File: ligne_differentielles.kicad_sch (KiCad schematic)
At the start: 2 parts, among them U16 AM26LS32ACDR

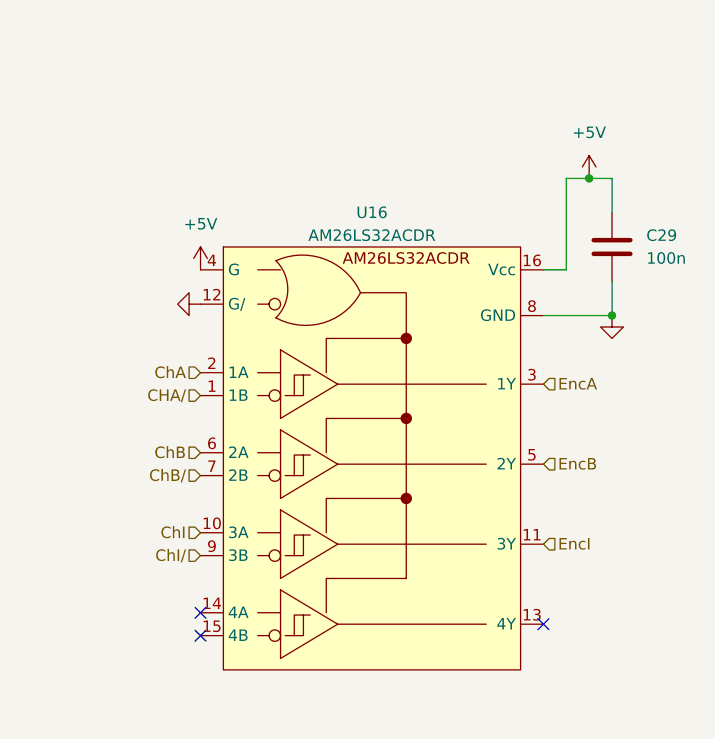
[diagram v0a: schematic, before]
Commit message: finalisation PCB
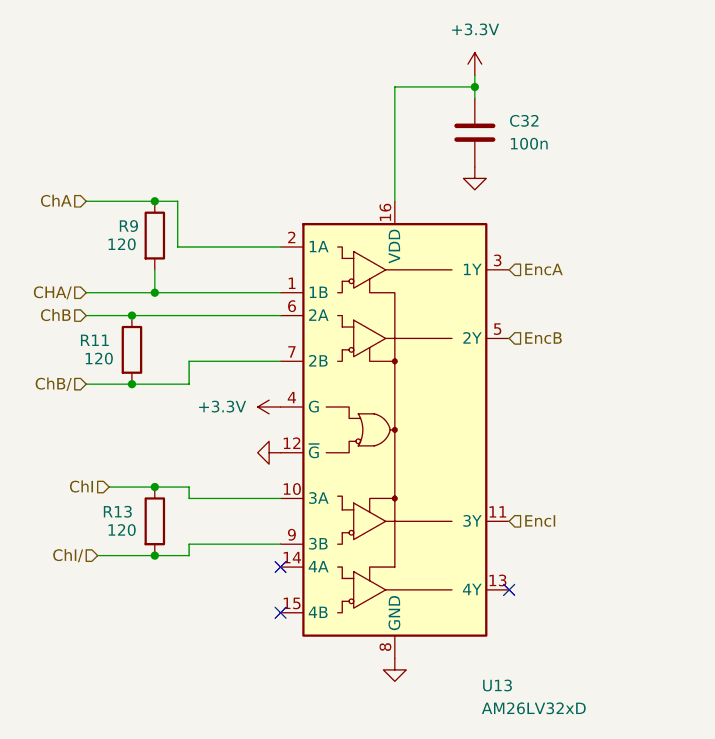
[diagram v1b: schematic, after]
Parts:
- removed C29: 100n, Capacitor_SMD:C_0402_1005Metric, symbol Device:C
- removed U16: AM26LS32ACDR, Package_SO:SOIC-16_3.9x9.9mm_P1.27mm, symbol AM26LS32Ax:AM26LS32ACDR
- added C32: 100n, Capacitor_SMD:C_0402_1005Metric, symbol Device:C
- added R11, R13, R9: 120, Resistor_SMD:R_0201_0603Metric, symbol Device:R
- added U13: AM26LV32xD, Package_SO:SOIC-16_3.9x9.9mm_P1.27mm, symbol Interface:AM26LV32xD
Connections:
- net CHA/: now also R9.2, U13.1 (1B)
- net ChA: now also R9.1, U13.2 (1A)
- net ChB: now also R11.1, U13.6 (2A)
- net ChB/: now also R11.2, U13.7 (2B)
- net ChI: now also R13.1, U13.10 (3A)
- net ChI/: now also R13.2, U13.9 (3B)
- net EncA: now also U13.3 (1Y)
- net EncB: now also U13.5 (2Y)
- net EncI: now also U13.11 (3Y)
- net GND: now also C32.2, U13.12 (~{G}), U13.8 (GND)
- new net +3.3V: C32.1, U13.16 (VDD), U13.4 (G)
